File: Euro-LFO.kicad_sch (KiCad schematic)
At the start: 32 parts, among them J1 Conn_02x05_Odd_Even, Q1 NPN, U1 TL074

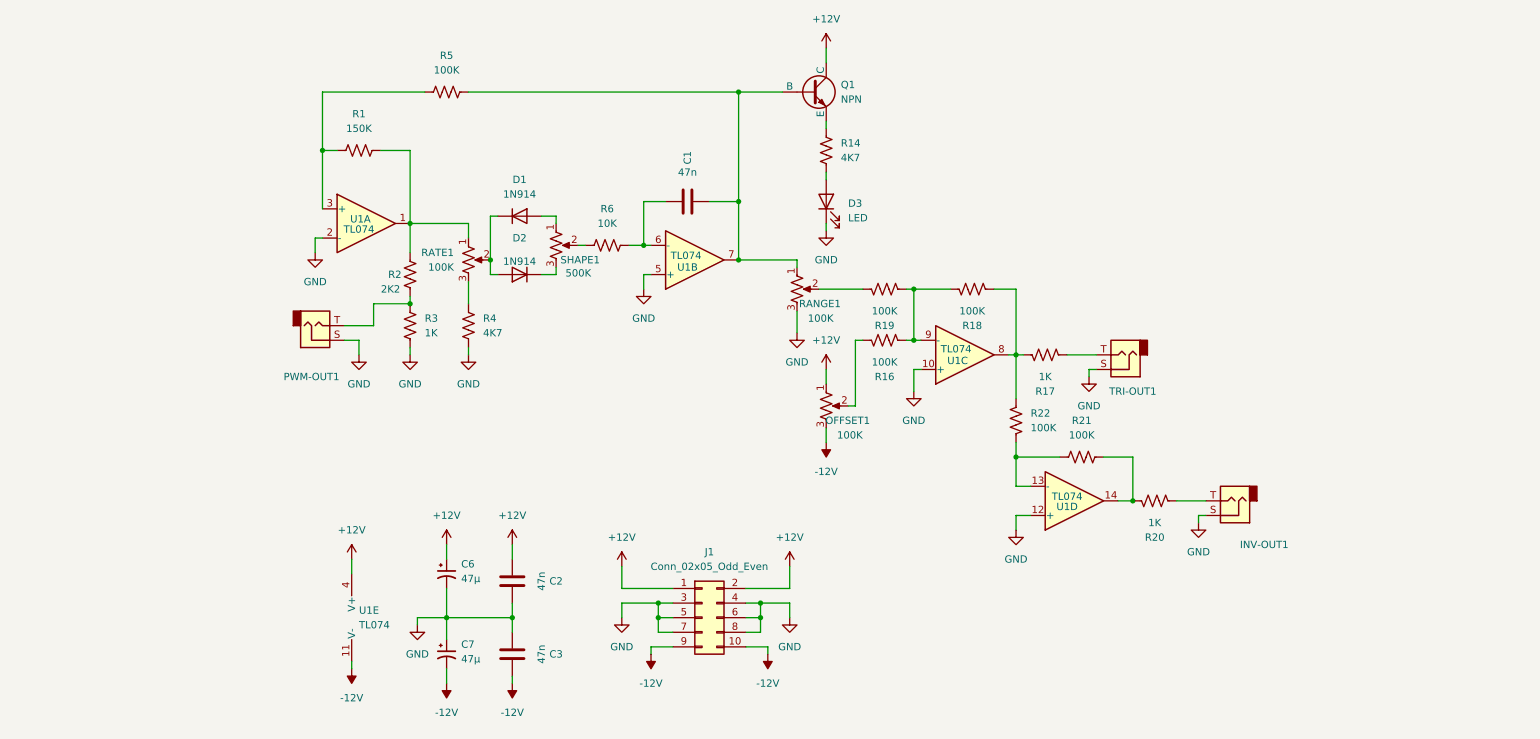
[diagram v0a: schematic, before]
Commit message: updated
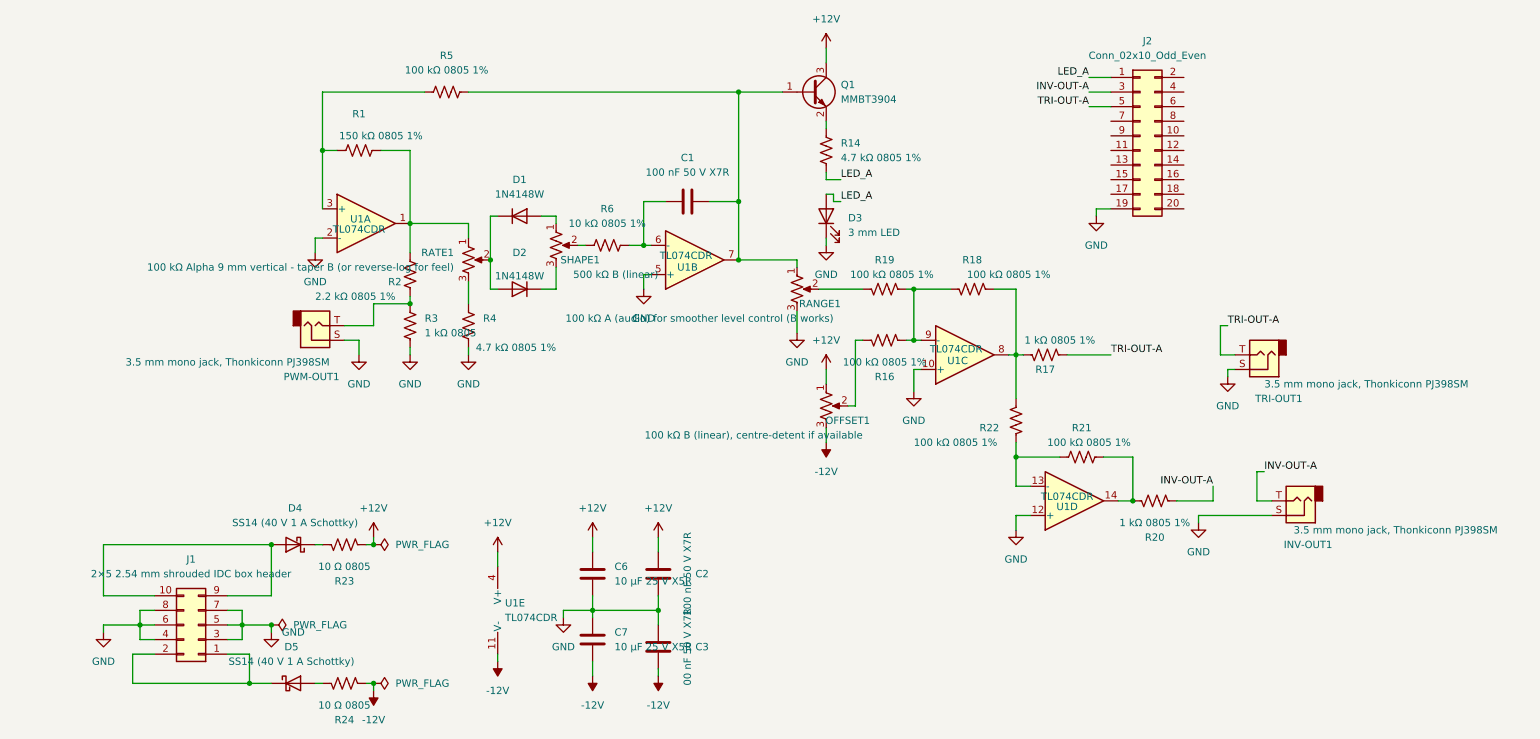
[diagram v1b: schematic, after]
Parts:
- removed Q1: NPN, Package_TO_SOT_SMD:SOT-23, symbol Simulation_SPICE:NPN
- added D4, D5: SS14 (40 V 1 A Schottky), Diode_SMD:D_SMA, symbol Device:D_Schottky
- added J2: Conn_02x10_Odd_Even, symbol Connector_Generic:Conn_02x10_Odd_Even
- added Q1: MMBT3904, Package_TO_SOT_SMD:SOT-23, symbol Transistor_BJT:MMBT3904
- added R23, R24: 10 Ω 0805, Resistor_SMD:R_0805_2012Metric, symbol Device:R_US
- C1, C2: value 47n -> 100 nF 50 V X7R; LCSC (none) -> C49678
- C3: value 47n -> 00 nF 50 V X7R; LCSC (none) -> C49678
- C6, C7: value 47µ -> 10 µF 25 V X5R; footprint (none) -> Capacitor_SMD:C_0805_2012Metric; symbol Device:C_Polarized_Small_US -> Device:C; LCSC (none) -> C15850
- D1, D2: value 1N914 -> 1N4148W; LCSC (none) -> C81598
- D3: value LED -> 3 mm LED
- INV-OUT1, PWM-OUT1, TRI-OUT1: value (none) -> 3.5 mm mono jack, Thonkiconn PJ398SM
- J1: value Conn_02x05_Odd_Even -> 2×5 2.54 mm shrouded IDC box header; footprint Connector_PinHeader_2.54mm:PinHeader_2x05_P2.54mm_Vertical -> Connector_IDC:IDC-Header_2x05_P2.54mm_Vertical
- OFFSET1: value 100K -> 100 kΩ B (linear), centre-detent if available
- R1: value 150K -> 150 kΩ 0805 1%; LCSC (none) -> C17557
- R14, R4: value 4K7 -> 4.7 kΩ 0805 1%; LCSC (none) -> C17673
- R16: value 100K -> 100 kΩ 0805 1%
- R17, R20: value 1K -> 1 kΩ 0805 1%; LCSC (none) -> C17513
- R18, R19, R21, R22, R5: value 100K -> 100 kΩ 0805 1%; LCSC (none) -> C149504
- R2: value 2K2 -> 2.2 kΩ 0805 1%; LCSC (none) -> C17726
- R3: value 1K -> 1 kΩ 0805; LCSC (none) -> C17513
- R6: value 10K -> 10 kΩ 0805 1%; LCSC (none) -> C17414
- RANGE1: value 100K -> 100 kΩ A (audio) for smoother level control (B works)
- RATE1: value 100K -> 100 kΩ Alpha 9 mm vertical - taper B (or reverse‑log for feel)
- SHAPE1: value 500K -> 500 kΩ B (linear)
- U1: value TL074 -> TL074CDR; LCSC (none) -> C6961
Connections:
- net +12V: now also Q1.3 (C), R23.1; no longer J1.1 (Pin_1), J1.2 (Pin_2)
- net -12V: now also R24.1; no longer J1.10 (Pin_10), J1.9 (Pin_9)
- net GND: now also J2.19 (Pin_19)
- net at R14.1: now also Q1.2 (E)
- net LED_A: now reaches D3.2 (A), R14.2
- net LED_A: now also J2.1 (Pin_1)
- net INV-OUT-A: now reaches INV-OUT1.T, R20.1
- net INV-OUT-A: now also J2.3 (Pin_3)
- net at C1.2, R5.1, RANGE1.1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: now also Q1.1 (B)
- net TRI-OUT-A: now reaches R17.1, TRI-OUT1.T
- net TRI-OUT-A: now also J2.5 (Pin_5)
- new net: D5.1 (K), J1.1 (Pin_1), J1.2 (Pin_2)
- new net: D5.2 (A), R24.2
- new net: D4.2 (A), J1.10 (Pin_10), J1.9 (Pin_9)
- new net: D4.1 (K), R23.2
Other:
- moved on the sheet: C2, C3, D2, D3, INV-OUT1, J1, TRI-OUT1, U1E
